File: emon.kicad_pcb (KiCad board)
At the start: 2 copper layers, 50.8 x 22.9 mm, 34 parts, among them J1 Screw_Terminal_01x02, J2 Conn_01x03_MountingPin, J3 USB_C_Receptacle_PowerOnly_6P, SW1 RESET, SW2 BOOTSEL, U1 RAK3172-T-8-SM-I, U2 BME690, U3 BQ25185

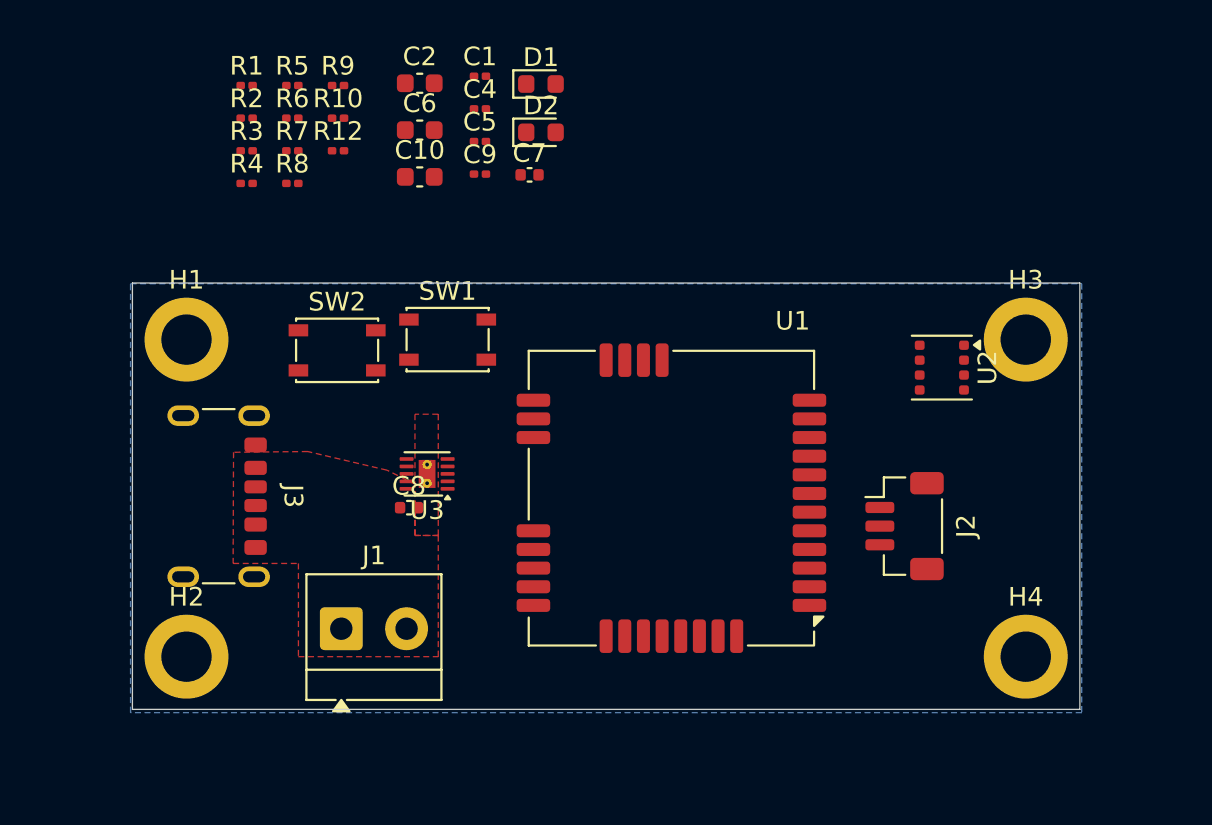
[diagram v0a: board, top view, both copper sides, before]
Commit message: layout progress
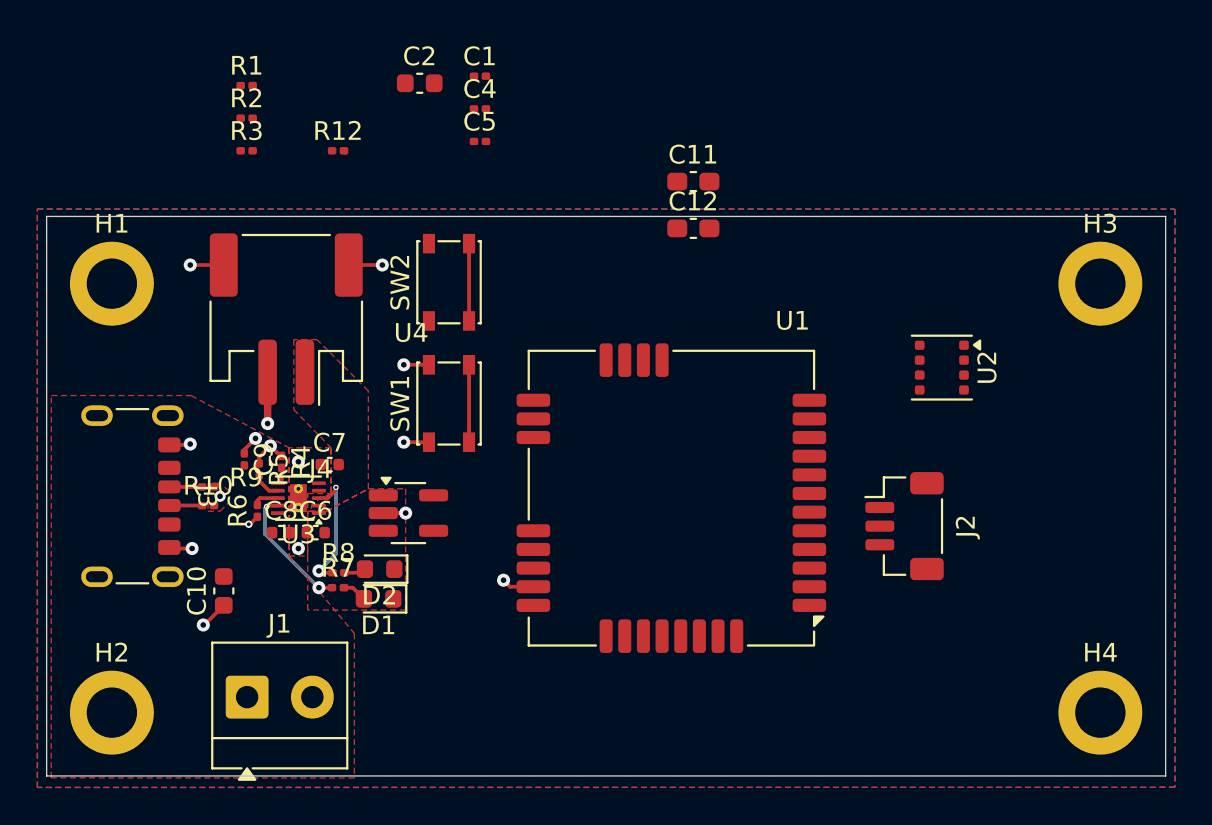
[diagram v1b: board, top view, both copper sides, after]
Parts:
- added C11: 1u, Capacitor_SMD:C_0603_1608Metric_Pad1.08x0.95mm_HandSolder, F.Cu at (153.2, 88.0)
- added C12: 1u, Capacitor_SMD:C_0603_1608Metric_Pad1.08x0.95mm_HandSolder, F.Cu at (153.2, 90.5)
- added J4: Conn_01x02_MountingPin, Connector_JST:JST_PH_S2B-PH-SM4-TB_1x02-1MP_P2.00mm_Horizontal, F.Cu at (131.3, 95.4)
- added U4: AP2112K-3.3, Package_TO_SOT_SMD:SOT-23-5_HandSoldering, F.Cu at (137.9, 105.8)
- C6: footprint Capacitor_SMD:C_0603_1608Metric -> Capacitor_SMD:C_0402_1005Metric
- moved D1 28.9 mm to (136.3, 110.4), turned to 180 degrees
- moved D2 25.0 mm to (136.4, 108.8), turned to 180 degrees
- moved C10 24.6 mm to (128.0, 110.0), turned to 90 degrees
- moved R7 23.6 mm to (134.1, 109.8)
- moved R9 22.6 mm to (127.2, 104.4)
- moved C6 22.3 mm to (132.9, 106.8)
- moved R10 21.9 mm to (127.2, 105.4)
- moved R6 21.1 mm to (129.8, 105.7), turned to 90 degrees
- moved R8 21.0 mm to (134.1, 109.0)
- moved R5 20.7 mm to (129.9, 103.5), turned to -90 degrees
- moved C9 19.8 mm to (129.1, 102.9), turned to -90 degrees
- moved C7 18.9 mm to (133.7, 103.2)
- moved R4 15.0 mm to (131.1, 103.1), turned to -90 degrees
- moved SW2 7.02 mm to (140.1, 93.4), turned to 90 degrees
- moved U3 7.02 mm to (132.0, 105.0)
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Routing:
- net GND: track 0.00 -> 19.6 mm, vias 0 -> 16
- net Net-(U3-STAT1): track 0.00 -> 6.92 mm, vias 0 -> 2
- net Net-(U3-STAT2): track 0.00 -> 6.84 mm, vias 0 -> 2
- net /BOOT: track 0.00 -> 4.95 mm
- net /RST: track 0.00 -> 4.15 mm
- net Net-(J3-CC2): track 0.00 -> 1.76 mm
- net Net-(J3-CC1): track 0.00 -> 1.76 mm
- net /ILIM/VSET: track 0.00 -> 1.52 mm
- net /ISET: track 0.00 -> 1.38 mm
- net Net-(D1-A): track 0.00 -> 1.32 mm
- net Net-(D2-A): track 0.00 -> 1.18 mm
- net /TS/MR: track 0.00 -> 0.91 mm
- added copper zone on F.Cu, net +3V3
- added copper zone on F.Cu, net +BATT
- added copper zone on F.Cu, net VDD
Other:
- board size 50.8 x 22.9 mm -> 60 x 30 mm
